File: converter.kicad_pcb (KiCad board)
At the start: 2 copper layers, 25.4 x 49.9 mm, 63 parts, among them CN1 MINI_DIN_8P_JACK, J1 USB_B, P1 CONN_1, P10 CONN_1, P11 CONN_1, P12 CONN_1, P13 CONN_1, P14 CONN_1, P15 CONN_1, P16 CONN_1, P17 CONN_1, P18 CONN_1, P19 CONN_1, P2 CONN_1, P20 CONN_1, P21 CONN_1, P22 CONN_1, P23 CONN_1, P24 CONN_1, P25 CONN_1, P26 CONN_1, P27 CONN_1, P28 CONN_1, P29 CONN_1, P3 CONN_1, P30 CONN_1, P31 CONN_1, P32 CONN_1, P33 CONN_1, P34 CONN_1, P35 CONN_1, P36 CONN_1, P37 CONN_1, P38 CONN_1, P39 CONN_1, P4 CONN_1, P40 CONN_1, P41 CONN_1, P42 CONN_1, P5 CONN_1, P6 CONN_1, P7 CONN_1, P8 CONN_1, P9 CONN_1, U1 ATMEGA32U4, X1 16MHz

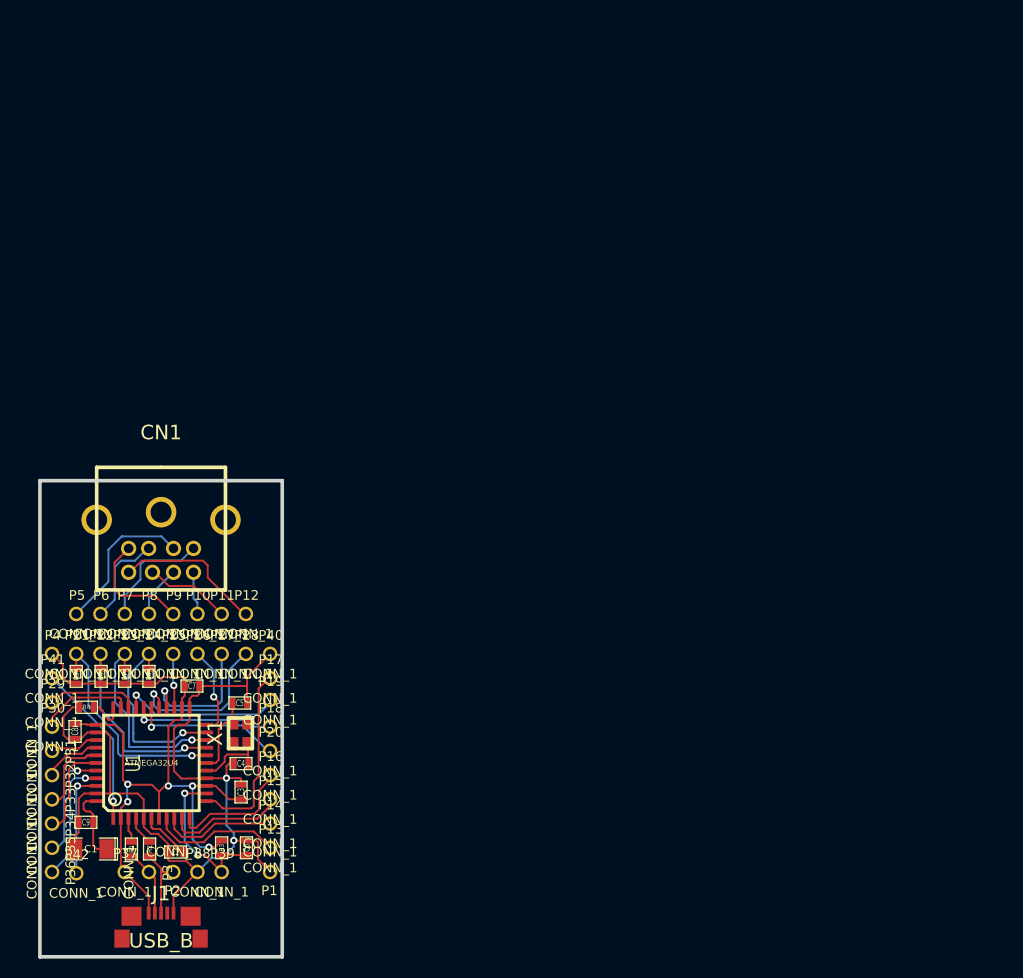
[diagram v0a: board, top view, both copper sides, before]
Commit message: Rev1 for fusion PCB
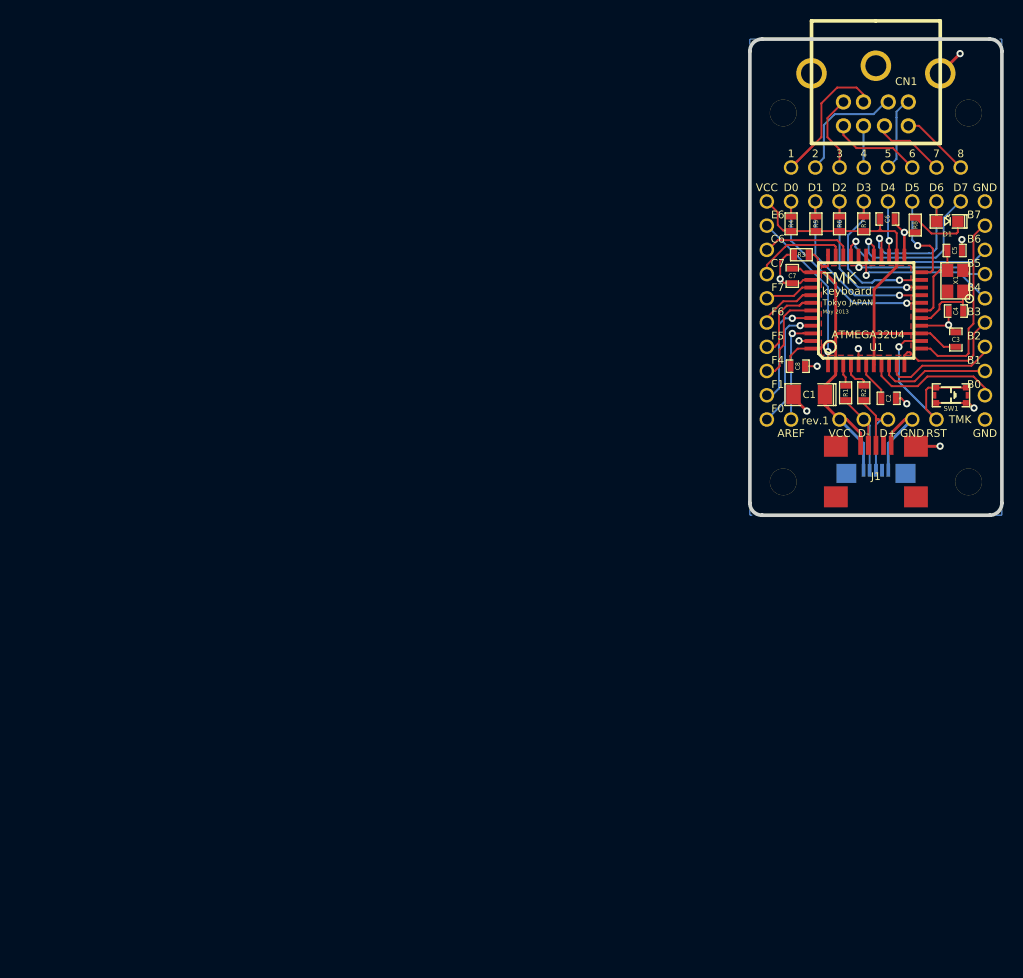
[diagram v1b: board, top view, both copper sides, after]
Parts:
- removed the C8 at (63.5, 150.7)
- removed P17, P19, P29, P41: CONN_1, PIN_1
- removed the R3 at (78.9, 162.9)
- added B6: CONN_1, PIN_1, F.Cu at (158.9, 100.3)
- added B7: CONN_1, PIN_1, F.Cu at (158.9, 97.7)
- added C7: 0.1u, SM0603_Capa, F.Cu at (138.7, 103.0)
- added D1: LED, LED_0805, F.Cu at (154.9, 97.3)
- added E6: CONN_1, PIN_1, F.Cu at (136.0, 97.7)
- added HOLE_M2.6: VAL**, HOLE_M2.6, F.Cu at (157.2, 124.6)
- added HOLE_M2.6: VAL**, HOLE_M2.6, F.Cu at (137.7, 85.9)
- added HOLE_M2.6: VAL**, HOLE_M2.6, F.Cu at (157.2, 85.9)
- added HOLE_M2.6: VAL**, HOLE_M2.6, F.Cu at (137.7, 124.6)
- added J2: USB_microB, USB_microB, B.Cu at (147.4, 126.0)
- added R8: 1K, SM0603, F.Cu at (151.6, 97.7)
- added SW1: SW_PUSH, SW_ALPS_SKSG, F.Cu at (155.3, 115.5)
- C6: value 0.1u -> CONN_1; footprint SM0603_Capa -> PIN_1
- J1: footprint USB_microB -> USB_miniB
- moved J1 89.5 mm to (147.4, 123.5)
- moved C1 89.1 mm to (140.5, 115.4)
- moved R1 88.8 mm to (144.3, 115.3)
- moved R2 88.8 mm to (146.2, 115.3)
- moved AREF 88.8 mm to (138.6, 118.0), turned to 180 degrees
- moved B1 88.7 mm to (158.9, 113.0)
- moved B5 88.7 mm to (158.9, 102.8)
- moved D1 88.7 mm to (141.1, 95.2)
- moved D2 88.7 mm to (143.6, 95.2)
- moved D4 88.7 mm to (148.7, 95.2)
- moved D5 88.7 mm to (151.3, 95.2)
- moved GND 88.7 mm to (158.9, 95.2)
- moved X1 88.7 mm to (155.8, 103.5)
- moved B0 88.7 mm to (158.9, 115.5)
- moved B2 88.7 mm to (158.9, 110.4)
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- renumbered P5 to 1, P6 to 2, P7 to 3, P8 to 4, P9 to 5, P10 to 6, P11 to 7, P12 to 8, P42 to AREF, P13 to B0, P14 to B1, P15 to B2, P16 to B3, P20 to B4, P18 to B5, C7 to C6, P30 to C7, C9 to C8, P2 to D+, P3 to D-, P21 to D0, P22 to D1, P23 to D2, P24 to D3, P25 to D4, P26 to D5, P27 to D6, P28 to D7, P36 to F0, P35 to F1, P34 to F4, P33 to F5, P32 to F6, P31 to F7, P1 to GND, P40 to GND, P38 to GND, R4 to R3, R5 to R4, R6 to R5, R7 to R6, R8 to R7, P39 to RST, P4 to VCC, P37 to VCC
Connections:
- C6 pad 1: /~RESET -> /PC6
- CN1 pad 11: (no net) -> GND
- J1 pad 7: (no net) -> GND
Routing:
- net GND: track 95.8 -> 51.3 mm, vias 2 -> 12
- net /DIN8: track 15.9 -> 7.30 mm
- net /~RESET: track 16.9 -> 25.2 mm, vias 2 -> 1
- net +5V: track 89.5 -> 83.0 mm, vias 5 -> 0
- net N-0000018: track 0.00 -> 6.31 mm
- net /D+: track 7.73 -> 13.3 mm
- net /DIN6: track 4.54 -> 9.59 mm
- net /D-: track 7.09 -> 11.3 mm
- net /DIN3: track 12.1 -> 8.09 mm
- net /DIN5: track 12.1 -> 8.30 mm
- net /PB2: track 15.1 -> 12.0 mm, vias 1 -> 0
- net /PD2: track 20.7 -> 18.0 mm
- net /DIN2: track 9.90 -> 12.6 mm
- net /PD6: track 14.4 -> 16.5 mm
- net N-0000022: track 5.93 -> 4.15 mm
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- added copper zone on F.Cu, net +5V
- added copper zone on B.Cu, net GND
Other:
- board size 25.4 x 49.9 mm -> 26.4 x 49.9 mm
- net class 12tho added: clearance 0.254, trace_width 0.3048, via_dia 0.762, via_drill 0.508
- net class 25tho removed
- net class 50tho removed
- rule via_min_size: 0.635 -> 0.762
- board text added: "May 2013"
- board text added: "TMK"
- board text added: "Tokyo JAPAN"
- board text added: "keyboard"
- board text added: "rev.1"
